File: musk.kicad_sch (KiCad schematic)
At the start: 56 parts, among them J1 debug-port, J10 Conn_01x06_Male, J3 Conn_01x06_Male, J4 Conn_01x06_Male, J5 Conn_01x06_Male, J6 Conn_01x06_Male, J7 Conn_01x06_Male, J8 Conn_01x06_Male, J9 Conn_01x06_Male, K1 diode-choc, K10 diode-choc, K11 diode-choc, K12 diode-choc, K13 diode-choc, K14 diode-choc, K15 diode-choc, K16 diode-choc, K2 diode-choc, K3 diode-choc, K4 diode-choc, K5 diode-choc, K6 diode-choc, K7 diode-choc, K8 diode-choc, K9 diode-choc, SW1 SW_Push, SW2 RotaryEncoder, U1 MT25QL128ABA1ESE, U2 ms88sf3-nrf52840, U3 LSM6DS3, U8 PMW3610, U9 MCP1804x-1802xMB

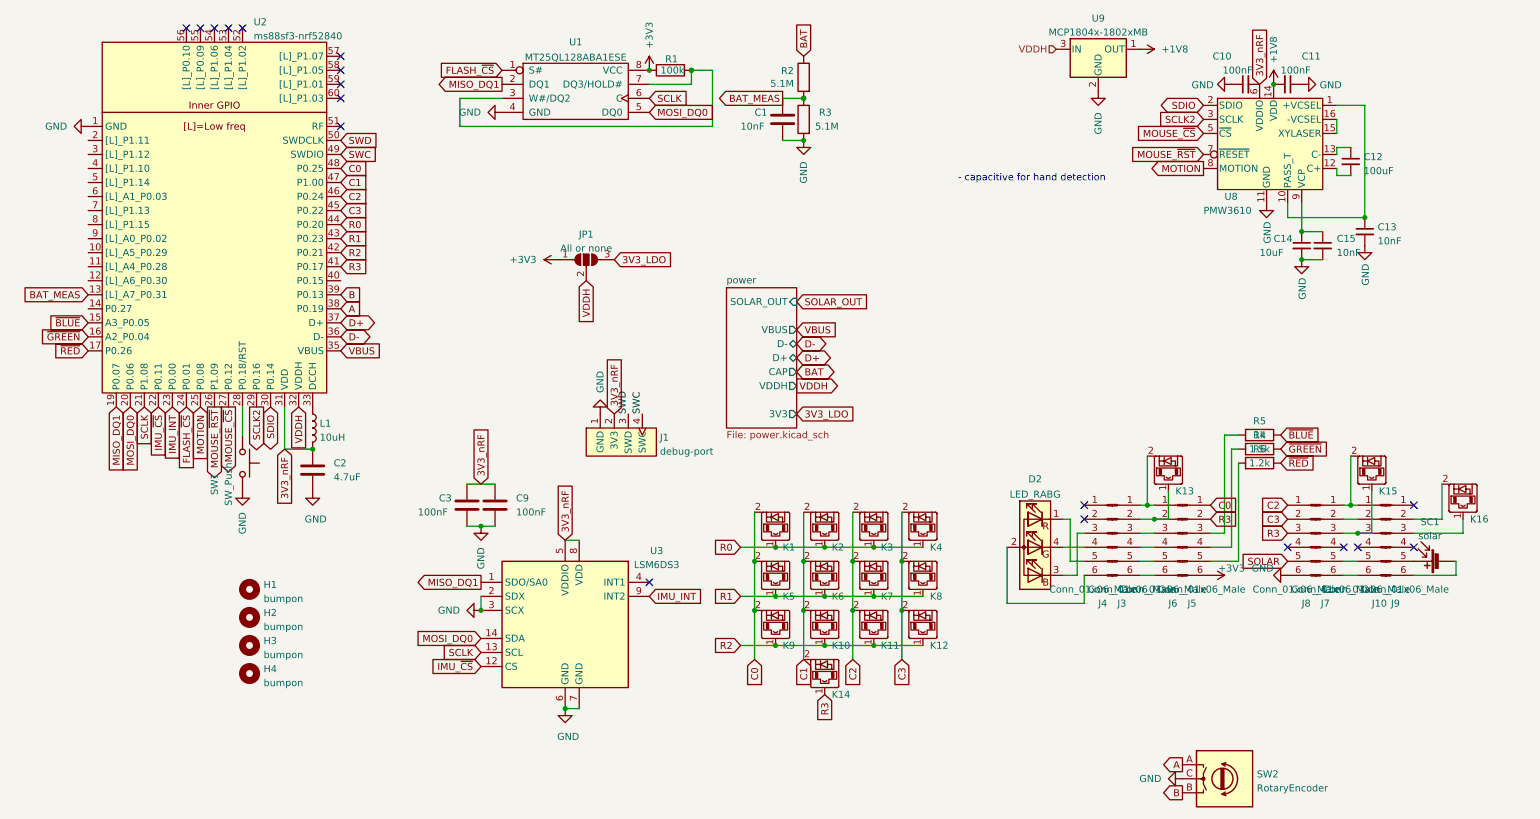
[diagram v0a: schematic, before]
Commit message: done
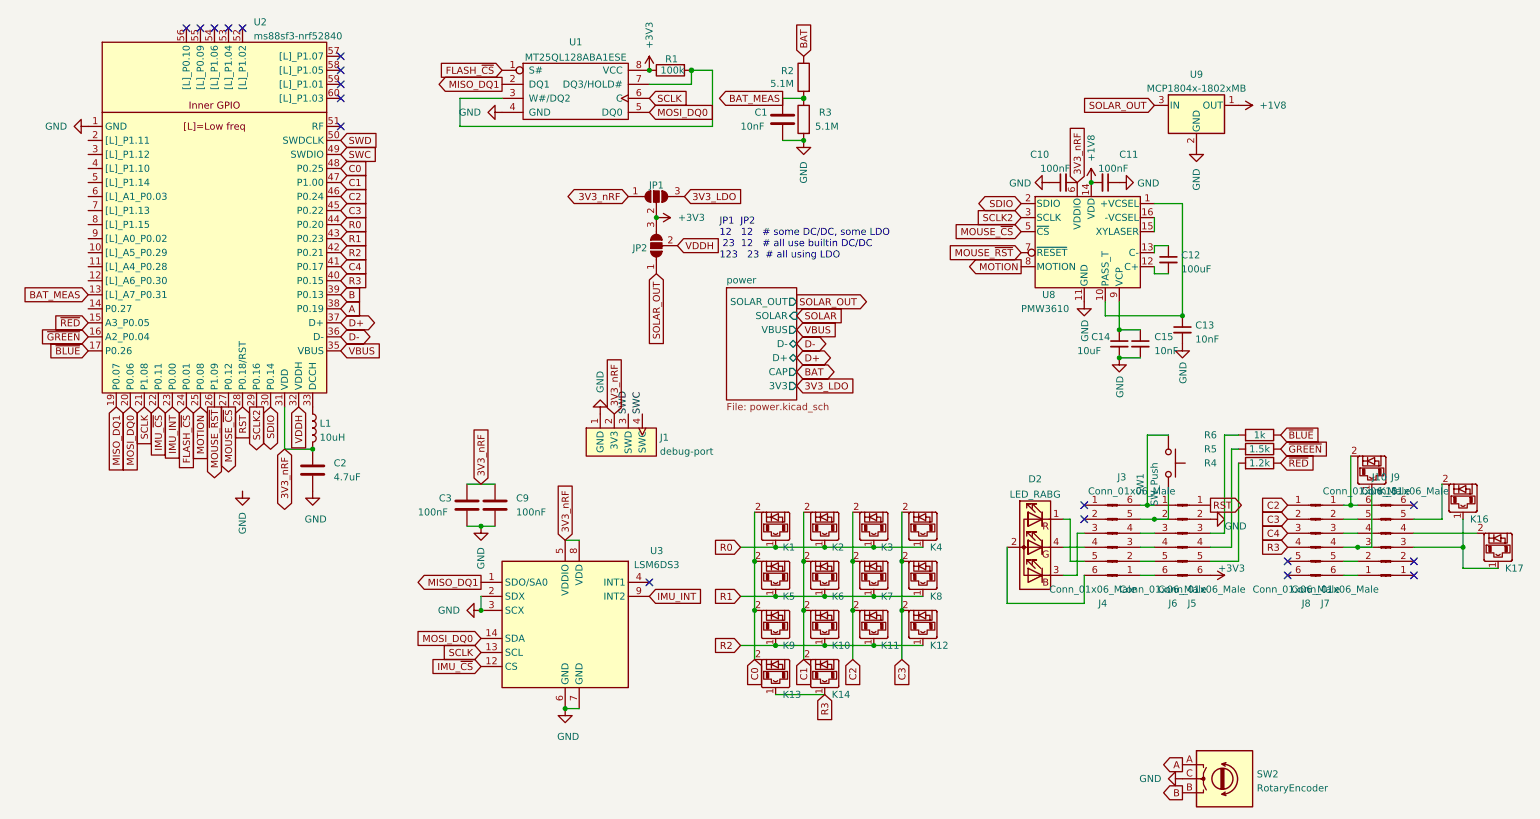
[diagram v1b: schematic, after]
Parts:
- removed H1, H2, H3, H4: bumpon, fusion:bumpon-sunk-hole, symbol Mechanical:MountingHole
- removed SC1: solar, misc:KXOB25-05X3F, symbol Device:Solar_Cell
- added JP2: left right or all, Jumper:SolderJumper-3_P1.3mm_Open_RoundedPad1.0x1.5mm, symbol Jumper:SolderJumper_3_Open
- added K17: diode-choc, pg1232:pg1232-DC, symbol switch:diode-choc
- JP1: value All or none -> left right or all
- K13: footprint pg1232:pg1232-DSS -> pg1232:pg1232-DC
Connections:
- net +3V3: now also JP1.2 (C), JP2.3 (B); no longer JP1.1 (A)
- net 3V3_nRF: now also JP1.1 (A)
- net C0: now also K13.2; no longer J5.1 (Pin_1)
- net GND: now also J5.2 (Pin_2); no longer J8.6 (Pin_6), SW1.2
- net R3: now also J8.4 (Pin_4), K13.1, U2.40 (P0.15); no longer J5.2 (Pin_2), J8.3 (Pin_3), U2.41 (P0.17)
- net SOLAR: no longer J8.5 (Pin_5)
- net SOLAR_OUT: now also U9.3 (IN), JP2.1 (A)
- net VDDH: now also JP2.2 (C); no longer JP1.2 (C), U9.3 (IN)
- net ~{BLUE}: now also U2.17 (P0.26); no longer U2.15 (A3_P0.05)
- net ~{RED}: now also U2.15 (A3_P0.05); no longer U2.17 (P0.26)
- net at J9.3 (Pin_3), K16.1: now also K17.1
- net at K16.2: now also J9.5 (Pin_5); no longer J9.2 (Pin_2)
- net at J3.3 (Pin_3): now also J6.4 (Pin_4); no longer J6.3 (Pin_3)
- net at J3.4 (Pin_4): now also J6.3 (Pin_3); no longer J6.4 (Pin_4)
- net at J6.5 (Pin_5): now also J3.2 (Pin_2); no longer J3.5 (Pin_5)
- net at J6.6 (Pin_6): now also J3.1 (Pin_1); no longer J3.6 (Pin_6)
- net at SW1.1: now also J3.6 (Pin_6), J6.1 (Pin_1); no longer U2.28 (P0.18/RST)
- net at J10.3 (Pin_3), K15.1: now also J7.4 (Pin_4); no longer J7.3 (Pin_3)
- net at J7.1 (Pin_1), K15.2: now also J10.6 (Pin_6); no longer J10.1 (Pin_1)
- net at J9.4 (Pin_4): now also K17.2
- net at J10.2 (Pin_2): now also J7.5 (Pin_5); no longer J7.2 (Pin_2)
- net at J10.4 (Pin_4): now also J7.3 (Pin_3)
- net at J10.5 (Pin_5): now also J7.2 (Pin_2); no longer J7.5 (Pin_5)
- net at J7.6 (Pin_6): now also J10.1 (Pin_1); no longer J10.6 (Pin_6)
- new net: J3.5 (Pin_5), J6.2 (Pin_2), SW1.2
- new net C4: J8.3 (Pin_3), U2.41 (P0.17)
- new net RST: J5.1 (Pin_1), U2.28 (P0.18/RST)
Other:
- sheet power ports: added SOLAR; removed VDDH
- note added: "JP1 JP2 12 12 # some DC/DC, some LDO 23 12 # all use builtin DC/DC 123 23 # all using LDO"
- note removed: "- capacitive for hand detection"
- moved on the sheet: C10, C11, C12, C13, C14, C15, J10, JP1, K13, SW1, U8, U9
